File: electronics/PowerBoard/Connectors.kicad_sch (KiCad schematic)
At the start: 7 parts, among them J401 Conn_02x20_Odd_Even, J402 PWR Stack, J404 PWR Stack, J405 Conn_01x04

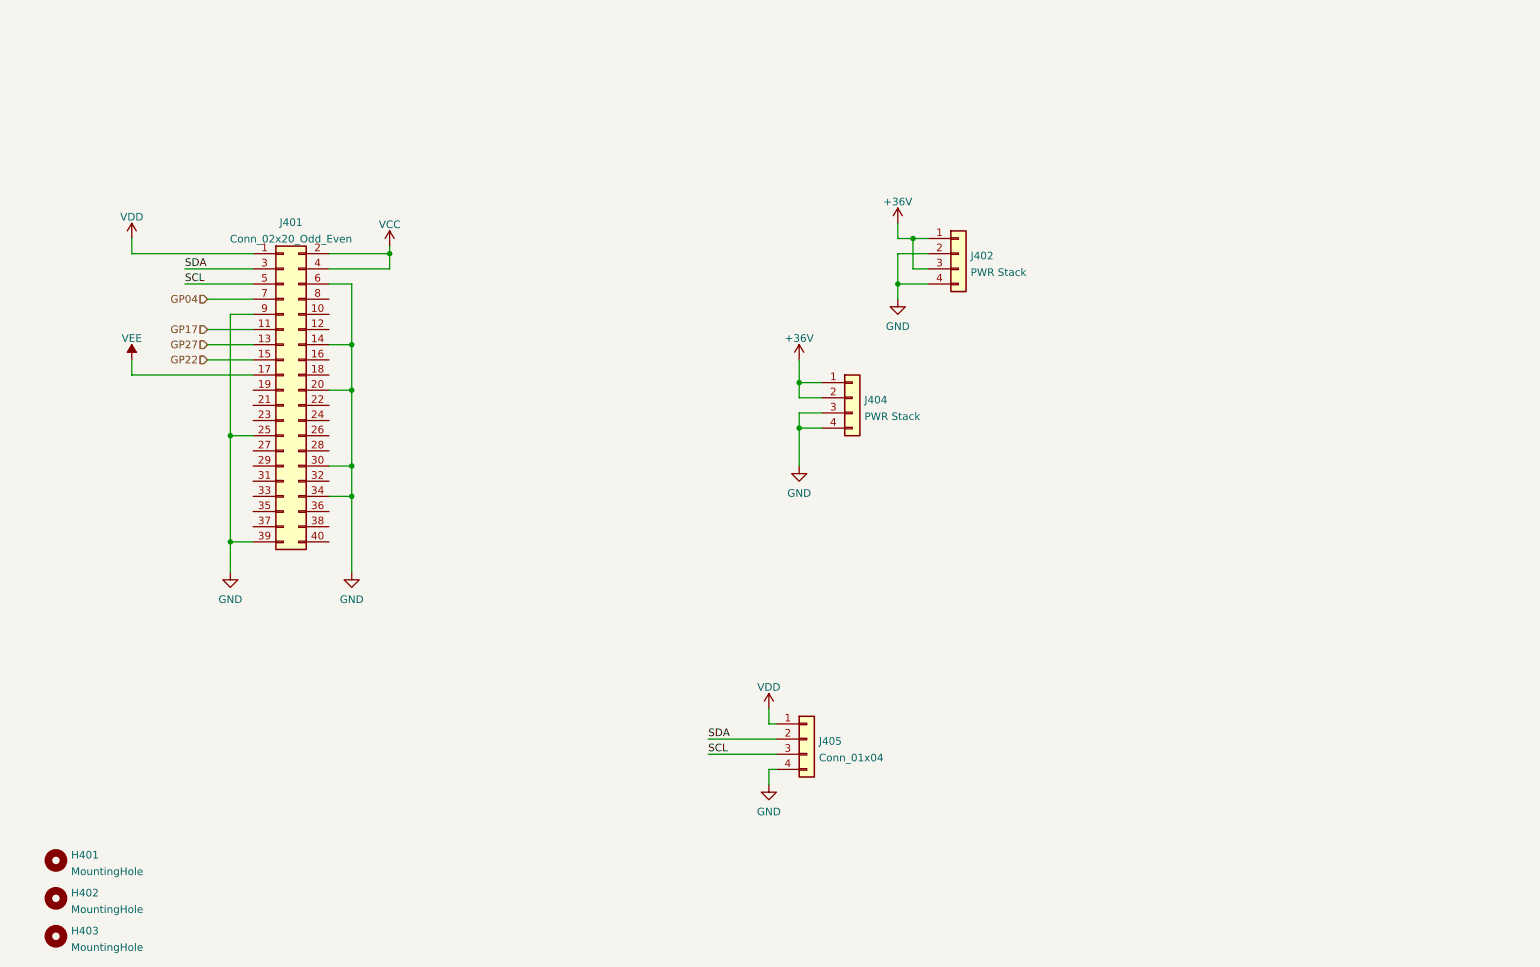
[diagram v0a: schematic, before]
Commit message: PowerBoard commit
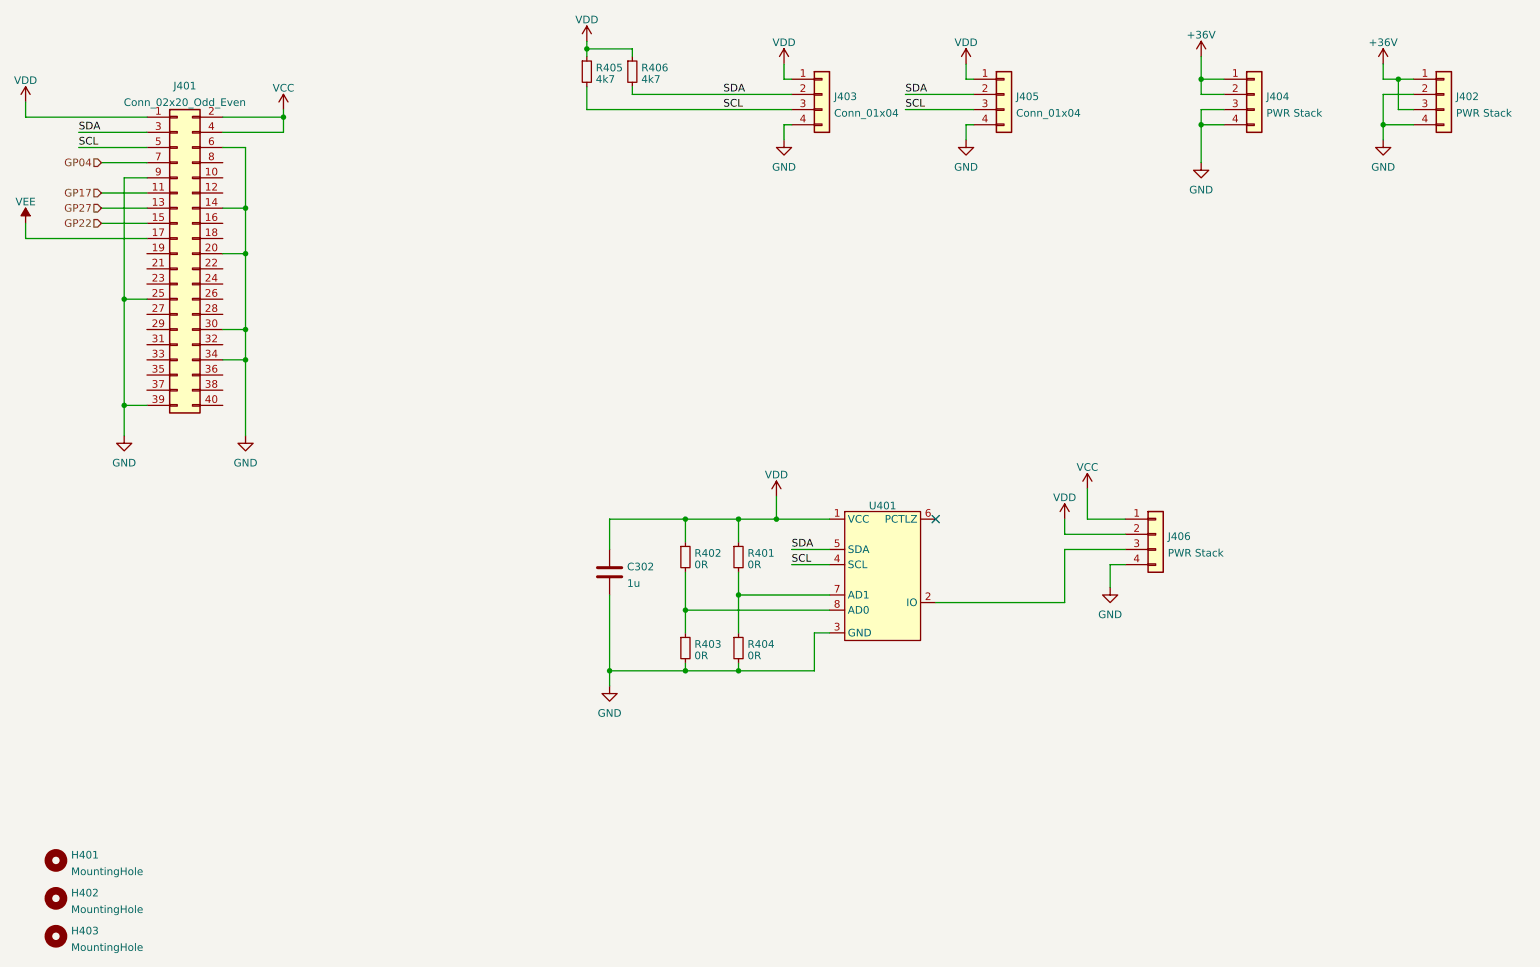
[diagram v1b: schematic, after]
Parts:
- added C302: 1u, Capacitor_SMD:C_0805_2012Metric, symbol Device:C
- added J403: Conn_01x04, Connector_PinSocket_2.54mm:PinSocket_1x04_P2.54mm_Vertical, symbol Connector_Generic:Conn_01x04
- added J406: PWR Stack, Connector_Phoenix_MC:PhoenixContact_MCV_1,5_4-G-3.5_1x04_P3.50mm_Vertical, symbol Connector_Generic:Conn_01x04
- added R401, R402, R403, R404: 0R, Resistor_SMD:R_0402_1005Metric, symbol Device:R_Small
- added R405, R406: 4k7, Resistor_SMD:R_0603_1608Metric, symbol Device:R_Small
- added U401: ~, Package_SO:SOIC-8_3.9x4.9mm_P1.27mm, symbol Findersee_parts:DS2482S-100+
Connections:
- net GND: now also C302.2, J403.4 (Pin_4), J406.4 (Pin_4), R403.2, R404.2, U401.3 (GND)
- net SCL: now also J403.3 (Pin_3), R405.2, U401.4 (SCL)
- net SDA: now also J403.2 (Pin_2), R406.2, U401.5 (SDA)
- net VCC: now also J406.1 (Pin_1)
- net VDD: now also C302.1, J403.1 (Pin_1), J406.2 (Pin_2), R401.1, R402.1, R405.1, R406.1, U401.1 (VCC)
- new net: J406.3 (Pin_3), U401.2 (IO)
- new net: R401.2, R404.1, U401.7 (AD1)
- new net: R402.2, R403.1, U401.8 (AD0)
- no-connect marks 0 -> 1
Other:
- moved on the sheet: J401, J402, J404, J405
